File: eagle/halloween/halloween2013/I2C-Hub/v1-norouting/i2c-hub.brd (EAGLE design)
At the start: 88.9 x 63.2 mm, 20 parts, among them J0 RJ12RIGHTANGLE-I2C, J1 RJ12RIGHTANGLE-I2C, J2 RJ12RIGHTANGLE-I2C, J3 RJ12RIGHTANGLE-I2C, J4 RJ12RIGHTANGLE-I2C, X1 87758-0616

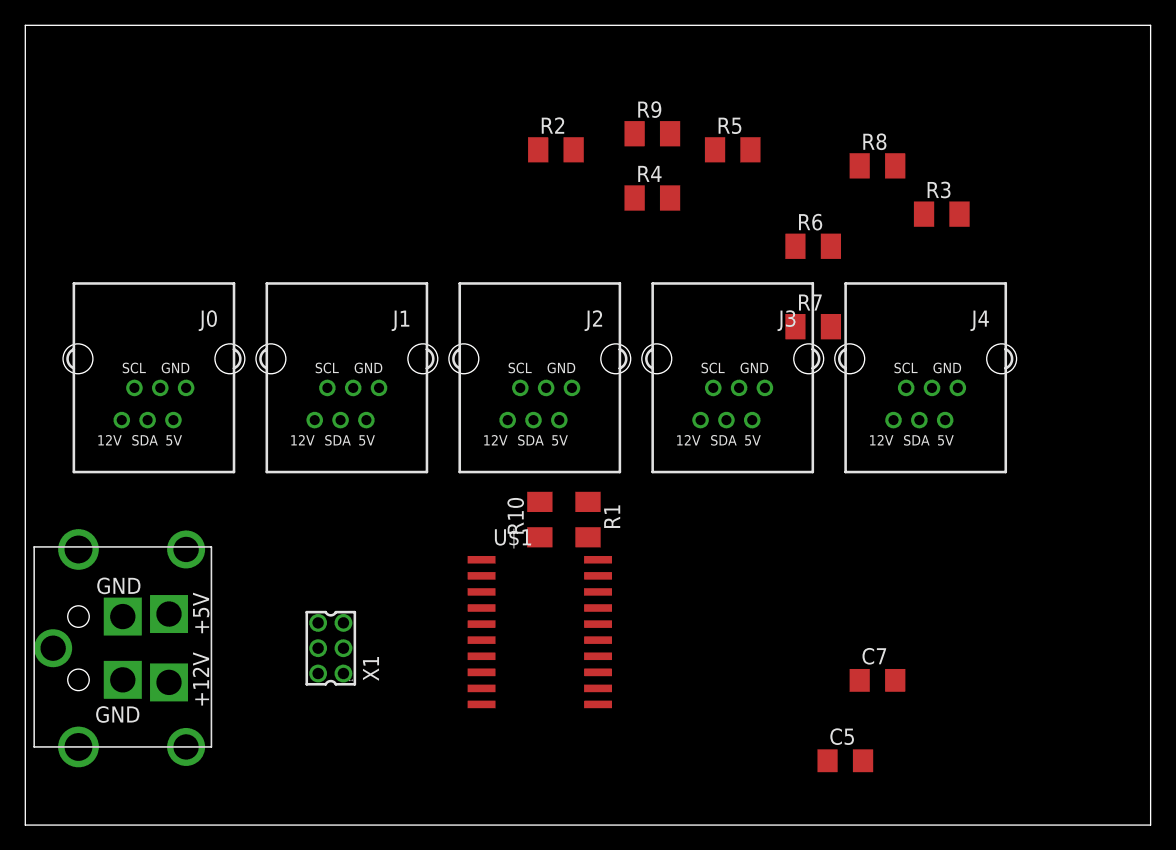
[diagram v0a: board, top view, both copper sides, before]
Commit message: Update halloween
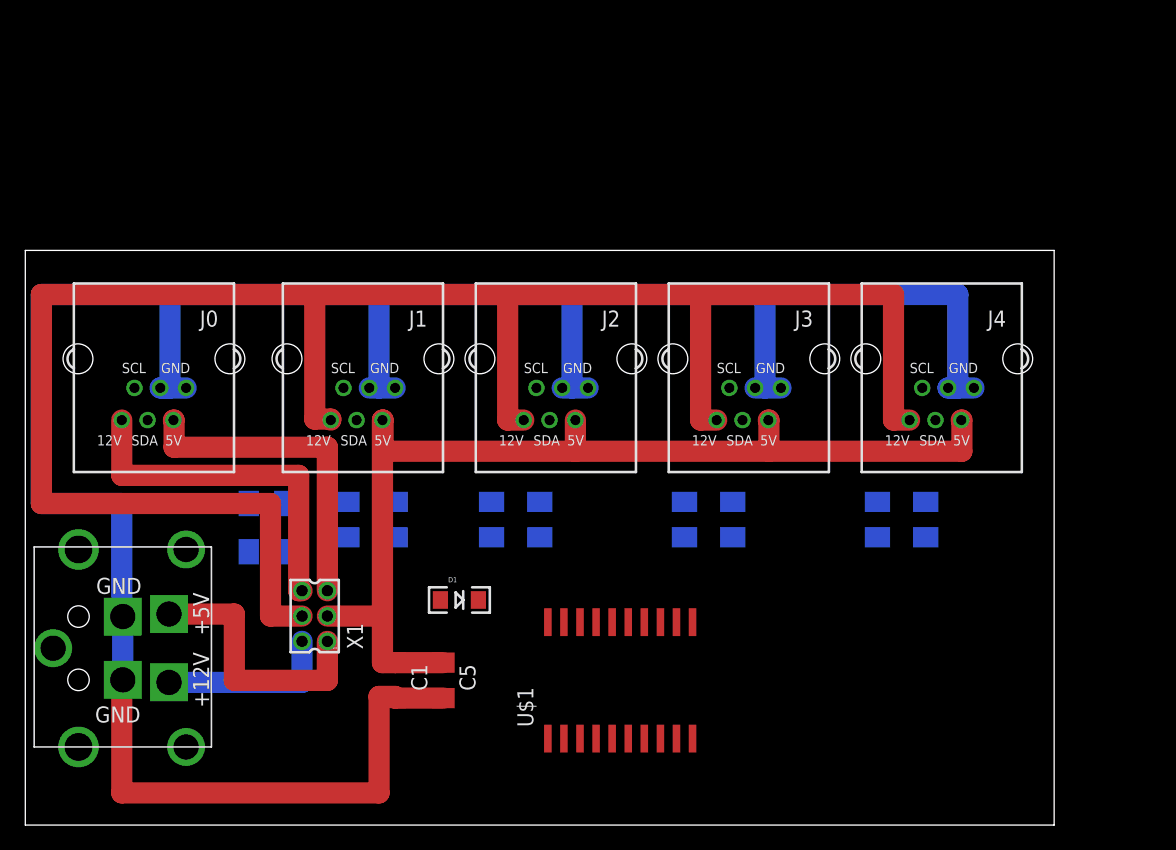
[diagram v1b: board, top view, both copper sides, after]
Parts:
- removed C7: 10uF, rcl:C1206
- added C1: 100nF, rcl:C1206
- added D1: 1N581D1206, lpatiny:LED-1206
- moved R8 47.2 mm to (29.2, 24.1), flipped to the bottom, turned to 270 degrees
- moved R5 42.2 mm to (25.4, 24.1), flipped to the bottom, turned to 90 degrees
- moved R2 36.1 mm to (19.1, 25.4), flipped to the bottom
- moved R9 33.0 mm to (36.8, 24.1), flipped to the bottom, turned to 270 degrees
- moved C5 32.4 mm to (33.0, 11.4), turned to 270 degrees
- moved R4 26.2 mm to (55.9, 24.1), flipped to the bottom, turned to 270 degrees
- moved R1 25.5 mm to (19.1, 21.6), flipped to the bottom, turned to 0 degrees
- moved R3 24.7 mm to (67.3, 24.1), flipped to the bottom, turned to 270 degrees
- moved R6 23.3 mm to (71.1, 24.1), flipped to the bottom, turned to 90 degrees
- moved R7 18.3 mm to (52.1, 24.1), flipped to the bottom, turned to 90 degrees
- moved U$1 7.41 mm to (47.0, 11.4), turned to 0 degrees
- moved X1 2.84 mm to (22.9, 16.5)
- moved J1 1.27 mm to (26.7, 36.8)
- moved J2 1.27 mm to (41.9, 36.8)
- moved J3 1.27 mm to (57.1, 36.8)
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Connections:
- removed net N$6: R8.2
- removed net VCC: U$1.20
- new net +5V1: D1.C, U$1.20
- net +12V: now also J1.+12V, J2.+12V, J3.+12V, J4.+12V
- net +5V: now also C1.1, C5.1, D1.A, J1.+5V, J2.+5V, J3.+5V, J4.+5V, R8.2
- net EXT-12V: no longer C7.2
- net EXT-5V: no longer C5.1
- net GND: now also C1.2; no longer C7.1
- net I2C-12V: no longer J1.+12V, J2.+12V, J3.+12V, J4.+12V
- net I2C-5V: no longer J1.+5V, J2.+5V, J3.+5V, J4.+5V
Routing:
- net GND: track 0.00 -> 200.0 mm
- net +12V: track 0.00 -> 158.1 mm
- net +5V: track 0.00 -> 84.0 mm
- net I2C-12V: track 0.00 -> 27.7 mm
- net I2C-5V: track 0.00 -> 25.6 mm
- net EXT-5V: track 0.00 -> 20.8 mm
- net EXT-12V: track 0.00 -> 13.8 mm
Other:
- board size 88.9 x 63.2 mm -> 81.3 x 45.4 mm
